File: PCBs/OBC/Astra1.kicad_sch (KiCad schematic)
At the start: 55 parts, among them J1 Conn_01x20, J2 Conn_01x20, J3 USB_C_Receptacle_USB2.0_16P, J4 Conn_01x04, J5 Conn_01x23, J6 Conn_01x23, J7 Conn_01x23, J8 Conn_01x23, SW1 SW_Push, SW2 SW_Push, SW3 SW_Push, U1 STM32F411CEUx, U2 W25Q32JVSS, U3 ME6231A33M3G, U4 DS3231M, Y1 32,768K, Y2 25MHz

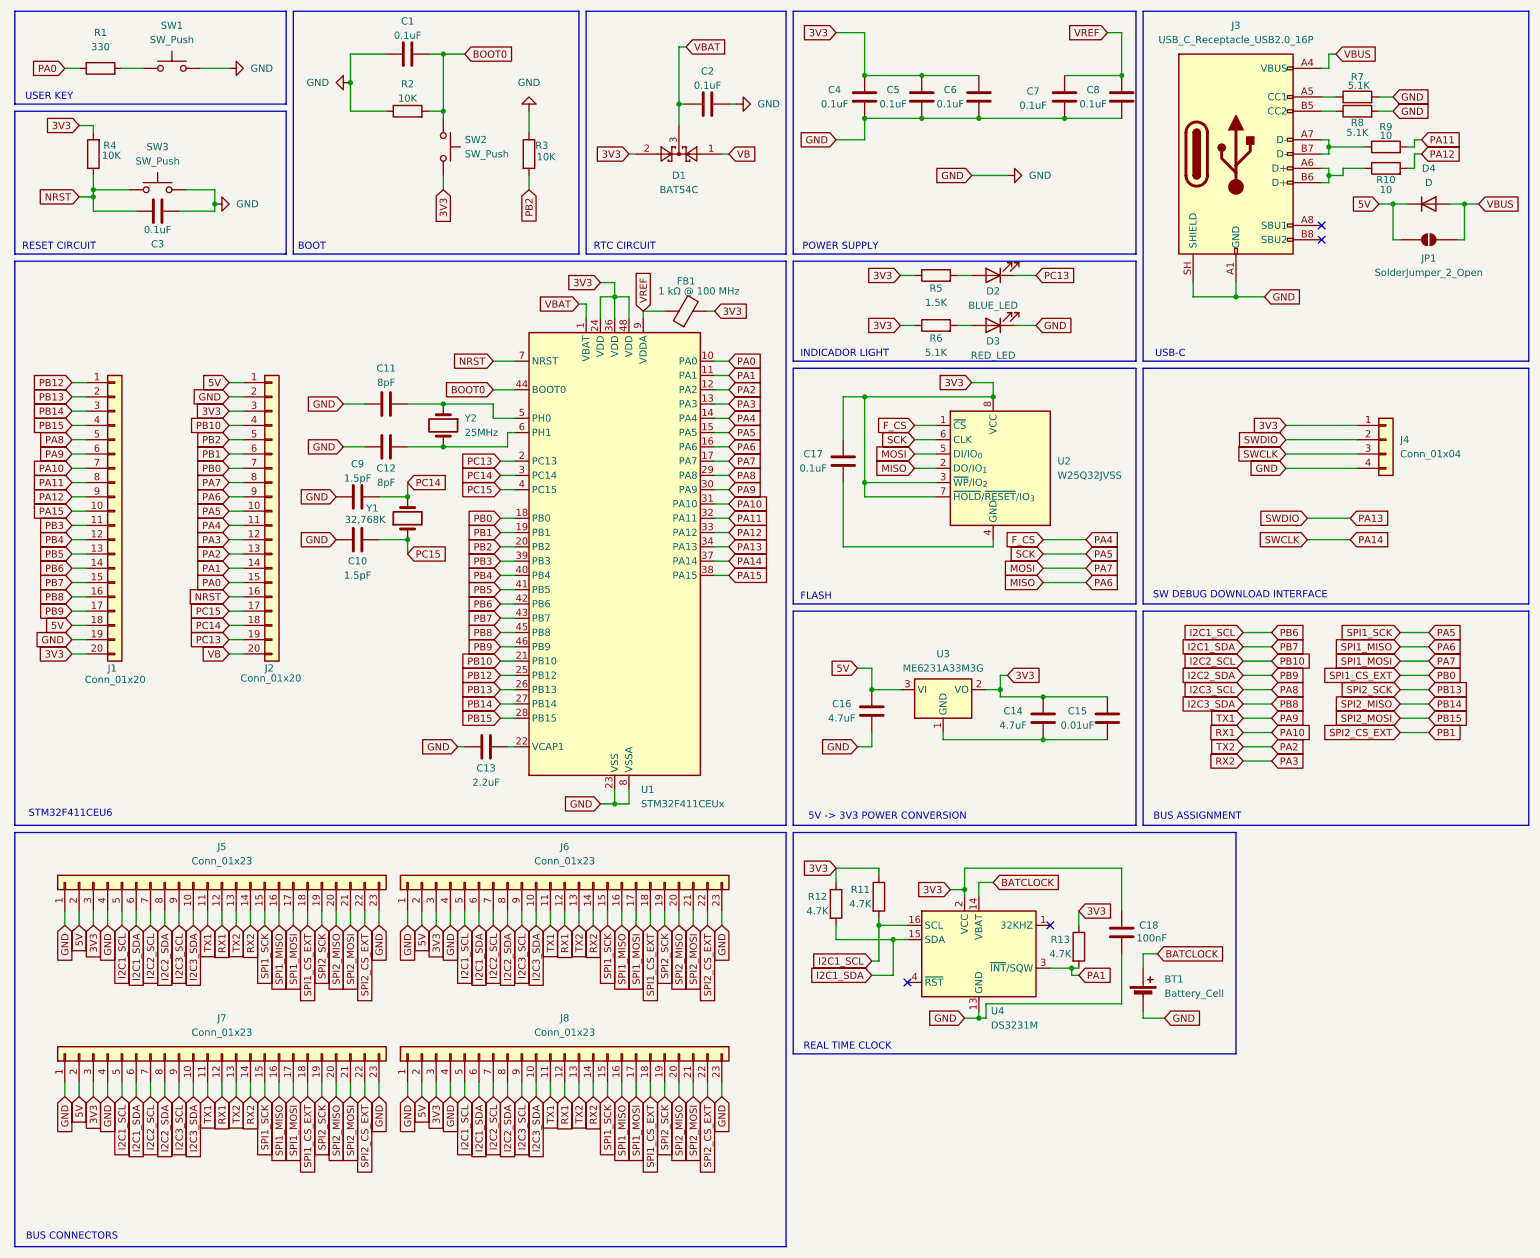
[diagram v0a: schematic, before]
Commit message: Avance de la segunda versión de la OBC
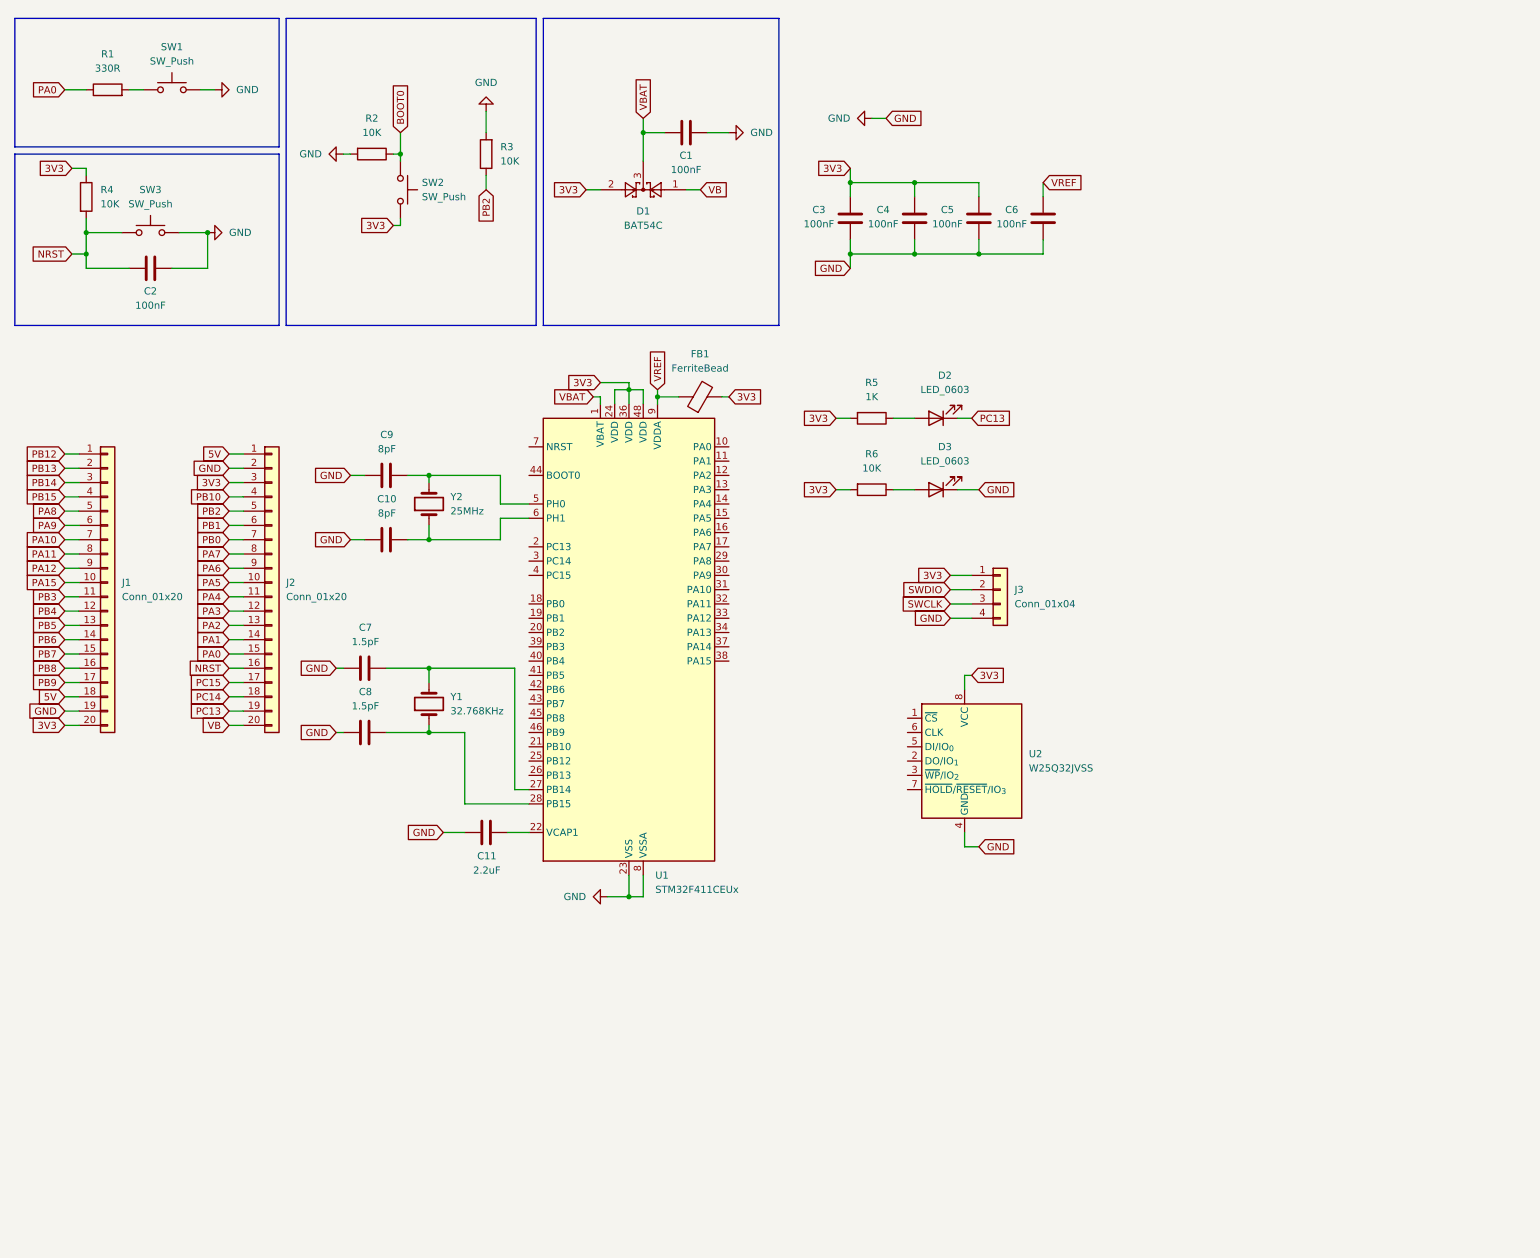
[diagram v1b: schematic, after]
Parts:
- removed BT1: Battery_Cell, Battery:BatteryHolder_Keystone_103_1x20mm, symbol Device:Battery_Cell
- removed C12: 8pF, Capacitor_SMD:C_0603_1608Metric, symbol Device:C
- removed C13: 2.2uF, Capacitor_SMD:C_0805_2012Metric, symbol Device:C
- removed C14, C16: 4.7uF, Capacitor_SMD:C_0805_2012Metric, symbol Device:C
- removed C15: 0.01uF, Capacitor_SMD:C_0603_1608Metric, symbol Device:C
- removed C17: 0.1uF, Capacitor_SMD:C_0603_1608Metric, symbol Device:C
- removed C18: 100nF, Capacitor_SMD:C_0805_2012Metric, symbol Device:C
- removed D4: D, Diode_SMD:D_SOD-323, symbol Device:D
- removed J3: USB_C_Receptacle_USB2.0_16P, Connector_USB:USB_C_Receptacle_HRO_TYPE-C-31-M-12, symbol Connector:USB_C_Receptacle_USB2.0_16P
- removed J4: Conn_01x04, Connector_PinHeader_2.54mm:PinHeader_1x04_P2.54mm_Horizontal, symbol Connector_Generic:Conn_01x04
- removed J5, J6, J7, J8: Conn_01x23, Connector_PinHeader_2.54mm:PinHeader_1x23_P2.54mm_Vertical, symbol Connector_Generic:Conn_01x23
- removed JP1: SolderJumper_2_Open, Jumper:SolderJumper-2_P1.3mm_Open_Pad1.0x1.5mm, symbol Jumper:SolderJumper_2_Open
- removed R10, R9: 10, Resistor_SMD:R_0603_1608Metric, symbol Device:R
- removed R11, R12, R13: 4.7K, Resistor_SMD:R_0603_1608Metric, symbol Device:R
- removed R7, R8: 5.1K, Resistor_SMD:R_0603_1608Metric, symbol Device:R
- removed U3: ME6231A33M3G, Package_TO_SOT_SMD:SOT-23-3, symbol Regulator_Linear:LD1117S33TR_SOT223
- removed U4: DS3231M, Package_SO:SOIC-16W_7.5x10.3mm_P1.27mm, symbol Timer_RTC:DS3231M
- added J3: Conn_01x04, symbol Connector_Generic:Conn_01x04
- C1, C2, C3, C4, C5, C6: value 0.1uF -> 100nF; footprint Capacitor_SMD:C_0603_1608Metric -> (none)
- C10, C9: value 1.5pF -> 8pF; footprint Capacitor_SMD:C_0603_1608Metric -> (none)
- C11: value 8pF -> 2.2uF; footprint Capacitor_SMD:C_0603_1608Metric -> (none)
- C7, C8: value 0.1uF -> 1.5pF; footprint Capacitor_SMD:C_0603_1608Metric -> (none)
- D1: footprint Package_TO_SOT_SMD:SOT-23-3 -> Package_TO_SOT_SMD:SOT-23
- D2: value BLUE_LED -> LED_0603; footprint LED_SMD:LED_0603_1608Metric -> (none)
- D3: value RED_LED -> LED_0603; footprint LED_SMD:LED_0603_1608Metric -> (none)
- FB1: value 1 kΩ @ 100 MHz -> FerriteBead; footprint Inductor_SMD:L_0603_1608Metric -> (none)
- J1, J2: footprint Connector_PinHeader_2.54mm:PinHeader_1x20_P2.54mm_Vertical -> (none)
- R1: value 330 -> 330R; footprint Resistor_SMD:R_0603_1608Metric -> (none)
- R2, R3, R4: footprint Resistor_SMD:R_0603_1608Metric -> (none)
- R5: value 1.5K -> 1K; footprint Resistor_SMD:R_0603_1608Metric -> (none)
- R6: value 5.1K -> 10K; footprint Resistor_SMD:R_0603_1608Metric -> (none)
- SW1, SW2, SW3: footprint Button_Switch_SMD:SW_SPST_PTS645Sx43SMTR92 -> (none)
- Y1: value 32,768K -> 32.768KHz; footprint Crystal:Crystal_SMD_3215-2Pin_3.2x1.5mm -> (none)
- Y2: footprint Crystal:Crystal_SMD_3225-4Pin_3.2x2.5mm -> (none)
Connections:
- net 3V3: now also C3.1, C4.1, C5.1, R4.1, R5.2, R6.2, J3.1 (Pin_1); no longer C4.2, C5.2, C6.2, R4.2, R5.1, R6.1, U2.3 (~{WP}/IO_{2}), U2.7 (~{HOLD}/~{RESET}/IO_{3})
- net BOOT0: now also R2.1; no longer C1.2, R2.2, U1.44 (BOOT0)
- net GND: now also C2.1, C3.2, C4.2, C5.2, C6.2, C7.2, C8.2, R2.2, R3.2, U2.4 (GND), J3.4 (Pin_4); no longer C2.2, C3.1, C4.1, C5.1, C6.1, C7.1, C8.1, R2.1, R3.1
- net NRST: now also C2.2, R4.2; no longer C3.2, R4.1, U1.7 (NRST)
- net PA0: no longer U1.10 (PA0)
- net PA1: no longer U1.11 (PA1)
- net PA10: no longer U1.31 (PA10)
- net PA11: no longer U1.32 (PA11)
- net PA12: no longer U1.33 (PA12)
- net PA15: no longer U1.38 (PA15)
- net PA2: no longer U1.12 (PA2)
- net PA3: no longer U1.13 (PA3)
- net PA5: no longer U1.15 (PA5), U2.6 (CLK)
- net PA9: no longer U1.30 (PA9)
- net PB0: no longer U1.18 (PB0)
- net PB1: no longer U1.19 (PB1)
- net PB12: no longer U1.25 (PB12)
- net PB13: no longer U1.26 (PB13)
- net PB14: no longer U1.27 (PB14)
- net PB15: no longer U1.28 (PB15)
- net PB2: now also R3.1; no longer R3.2, U1.20 (PB2)
- net PB3: no longer U1.39 (PB3)
- net PB4: no longer U1.40 (PB4)
- net PB5: no longer U1.41 (PB5)
- net PC13: no longer U1.2 (PC13)
- net PC14: no longer C9.1, U1.3 (PC14), Y1.2
- net PC15: no longer C10.1, U1.4 (PC15), Y1.1
- net VBAT: now also C1.2; no longer C2.1
- net VREF: now also C6.1; no longer C7.2, C8.2
- net at Y2.2: now also C9.1, U1.5 (PH0); no longer U1.6 (PH1)
- net at U1.22 (VCAP1): now also C11.2
- net at D2.2 (A): now also R5.1; no longer R5.2
- net at D3.2 (A): now also R6.1; no longer R6.2
- removed net F_CS: J2.11 (Pin_11), U1.14 (PA4), U2.1 (~{CS})
- net I2C1_SCL: no longer names the net of U1.42 (PB6)
- net I2C1_SCL: no longer J1.14 (Pin_14)
- net I2C1_SDA: no longer names the net of U1.43 (PB7)
- net I2C1_SDA: no longer J1.15 (Pin_15)
- net I2C2_SCL: no longer names the net of U1.21 (PB10)
- net I2C2_SCL: no longer J2.4 (Pin_4)
- net I2C2_SDA: no longer names the net of U1.46 (PB9)
- net I2C2_SDA: no longer J1.17 (Pin_17)
- net I2C3_SCL: no longer names the net of U1.29 (PA8)
- net I2C3_SCL: no longer J1.5 (Pin_5)
- net I2C3_SDA: no longer names the net of U1.45 (PB8)
- net I2C3_SDA: no longer J1.16 (Pin_16)
- removed net MISO: J2.9 (Pin_9), U1.16 (PA6), U2.2 (DO/IO_{1})
- removed net MOSI: J2.8 (Pin_8), U1.17 (PA7), U2.5 (DI/IO_{0})
- net PA13: no longer names the net of U1.34 (PA13)
- net PA14: no longer names the net of U1.37 (PA14)
- new net: C8.1, U1.28 (PB15), Y1.1
- new net: C10.1, U1.6 (PH1), Y2.1
- new net: C7.1, U1.27 (PB14), Y1.2
- new net PA4: J2.11 (Pin_11)
- new net PA6: J2.9 (Pin_9)
- new net PA7: J2.8 (Pin_8)
- new net PA8: J1.5 (Pin_5)
- new net PB10: J2.4 (Pin_4)
- new net PB6: J1.14 (Pin_14)
- new net PB7: J1.15 (Pin_15)
- new net PB8: J1.16 (Pin_16)
- new net PB9: J1.17 (Pin_17)
- new net SWCLK: J3.3 (Pin_3)
- new net SWDIO: J3.2 (Pin_2)
- no-connect marks 4 -> 0
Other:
- note removed: "5V -> 3V3 POWER CONVERSION"
- note removed: "BOOT"
- note removed: "BUS ASSIGNMENT"
- note removed: "BUS CONNECTORS"
- note removed: "FLASH"
- note removed: "INDICADOR LIGHT"
- note removed: "POWER SUPPLY"
- note removed: "REAL TIME CLOCK"
- note removed: "RESET CIRCUIT"
- note removed: "RTC CIRCUIT"
- note removed: "STM32F411CEU6"
- note removed: "SW DEBUG DOWNLOAD INTERFACE"
- note removed: "USB-C"
- note removed: "USER KEY"
